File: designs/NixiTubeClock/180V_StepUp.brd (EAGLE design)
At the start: 54 x 40 mm, 14 parts, among them IC1 MAX1771, Q1 RF644, X1 332-08

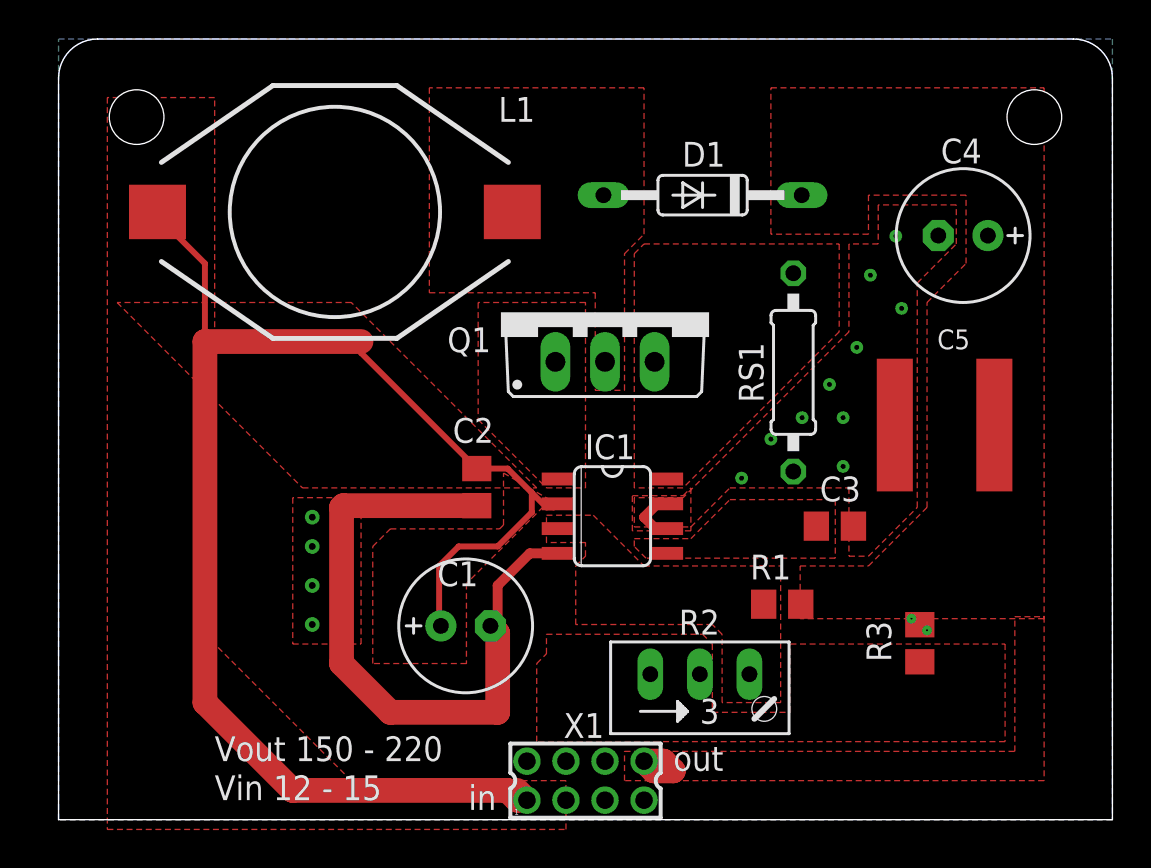
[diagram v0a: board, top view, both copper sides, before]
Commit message: started work on mainboard
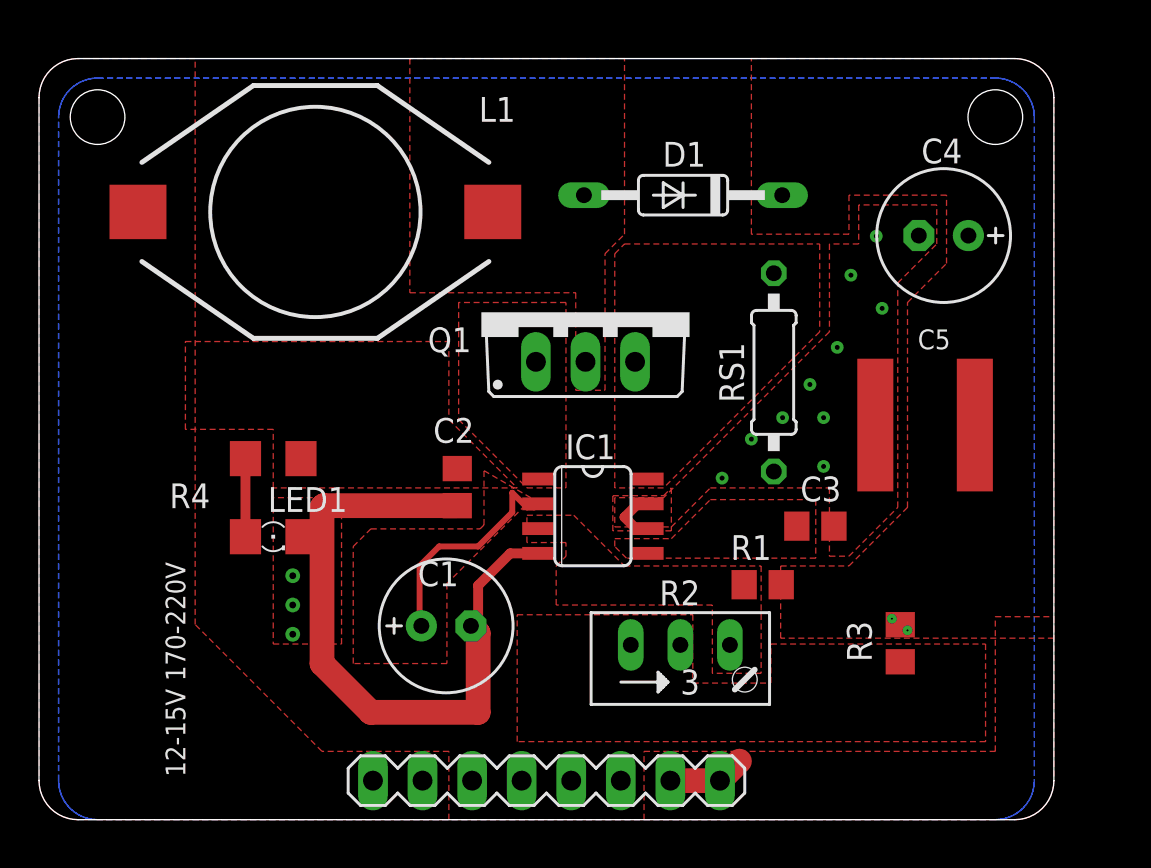
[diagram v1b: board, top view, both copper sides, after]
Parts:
- removed X1: 332-08, con-garry:332-08
- added LED1: GREEN, CommonParts:1206
- added R4: 1K, CommonParts:R1206
- added SV2: (no value), con-lstb:MA08-1
- moved R2 1.80 mm to (31.9, 8.32)
- moved R1 1.41 mm to (36.1, 12.0)
- moved C1 1.00 mm to (19.9, 9.93)
- moved C2 1.00 mm to (20.4, 17.0)
- moved C3 1.00 mm to (38.8, 15.0)
- moved C4 1.00 mm to (45.4, 29.9)
- moved C5 1.00 mm to (44.4, 20.2)
- moved D1 1.00 mm to (32.0, 32.0)
- moved IC1 1.00 mm to (27.4, 15.6)
- moved L1 1.00 mm to (13.2, 31.1)
- moved Q1 1.00 mm to (27.0, 26.0)
- moved R3 1.00 mm to (43.1, 9.04)
- moved RS1 1.00 mm to (36.6, 22.9)
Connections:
- new net N$1: LED1.A, R4.2
- net +170V: now also SV2.7, SV2.8; no longer X1.8
- net GND: now also LED1.C, SV2.3, SV2.4, SV2.5, SV2.6; no longer X1.2, X1.3, X1.4, X1.5, X1.6, X1.7
- net VIN: now also R4.1, SV2.1, SV2.2; no longer X1.1
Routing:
- net VIN: track 78.2 -> 12.5 mm
- net N$1: track 0.00 -> 4.00 mm
- net +170V: track 3.41 -> 3.95 mm
- net GND: vias 16 -> 15
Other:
- board size 54 x 40 mm -> 52 x 39 mm
- board text added: "12-15V 170-220V"
- board text added: "12V"
- board text added: "170V"
- board text added: "GND"
- board text removed: "Vin 12 - 15"
- board text removed: "Vout 150 - 220"
- board text removed: "in"
- board text removed: "out"
